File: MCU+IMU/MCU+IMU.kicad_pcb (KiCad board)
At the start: 4 copper layers, 32.8 x 32.8 mm, 21 parts, among them J1 Conn_01x04_Male, SW1 SW_Push, U1 LSM6DSV16XTR, U2 STM32F091RCT6, U3 RN4871, U4 MAX7375AXR405

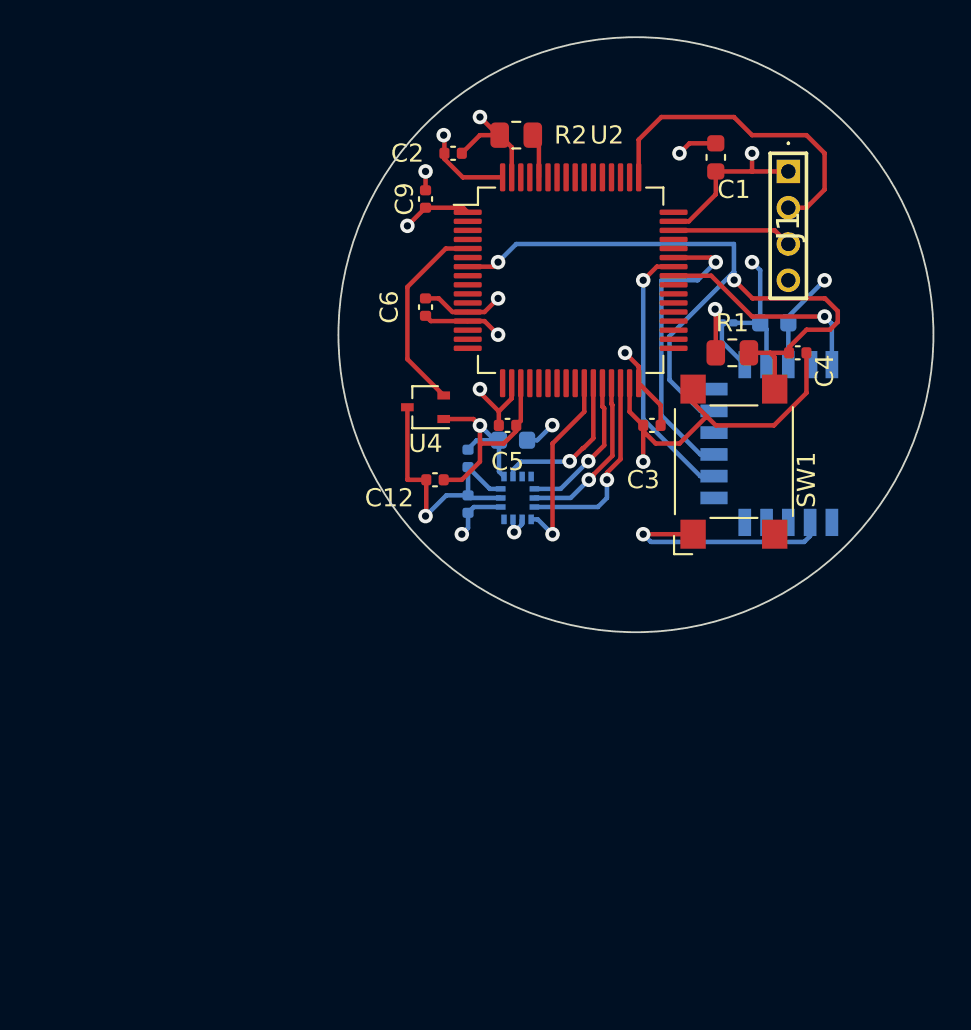
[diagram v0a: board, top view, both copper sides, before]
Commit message: Ordered
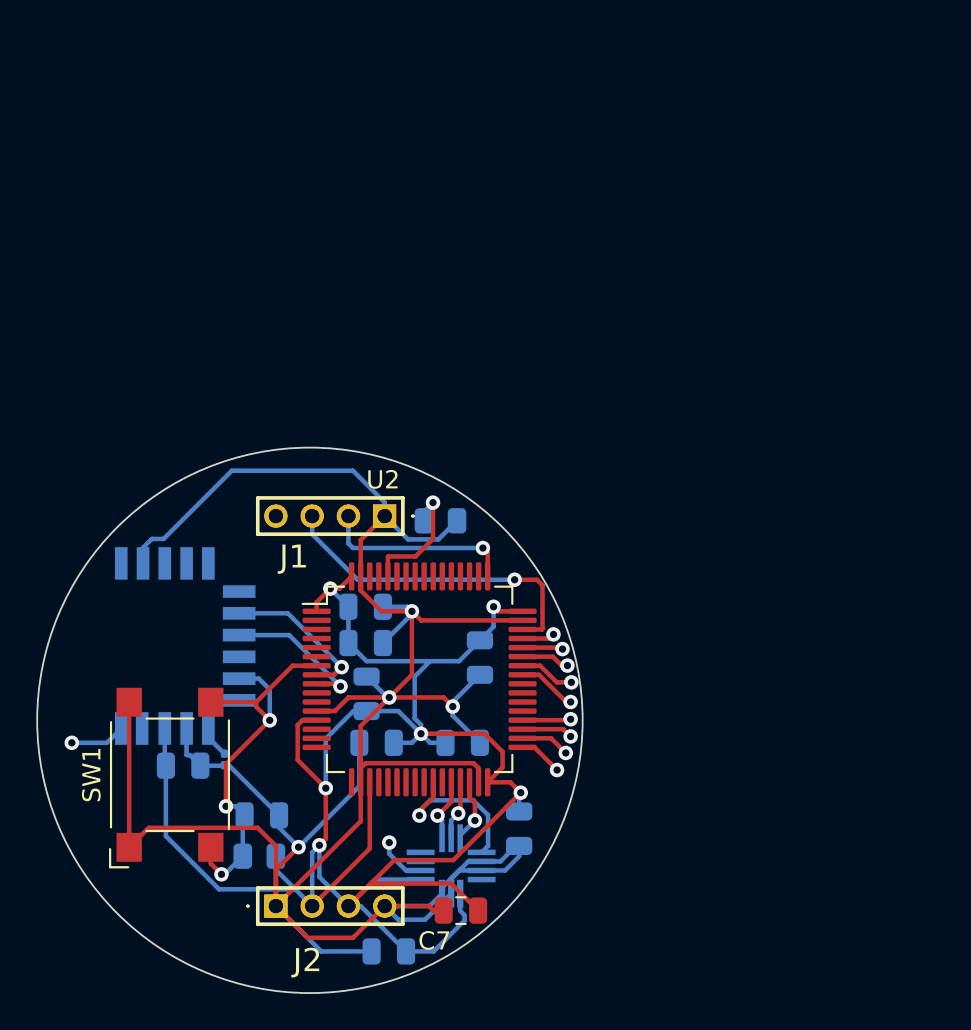
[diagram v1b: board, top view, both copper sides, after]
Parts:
- removed C12: 100n, Capacitor_SMD:C_0402_1005Metric
- removed U4: MAX7375AXR405, Package_TO_SOT_SMD:SOT-323_SC-70
- added J2: Conn_01x04_Male, 4PinConnector:2MMHBS04VT02HTB, F.Cu at (129.8, 113.5)
- C1: footprint Capacitor_SMD:C_0603_1608Metric -> Capacitor_SMD:C_0805_2012Metric; moved to B.Cu
- C10, C11: footprint Capacitor_SMD:C_0603_1608Metric -> Capacitor_SMD:C_0805_2012Metric
- C2, C3, C4, C5, C6, C9: footprint Capacitor_SMD:C_0402_1005Metric -> Capacitor_SMD:C_0805_2012Metric; moved to B.Cu
- C7: footprint Capacitor_SMD:C_0402_1005Metric -> Capacitor_SMD:C_0805_2012Metric; moved to F.Cu
- C8: footprint Capacitor_SMD:C_0402_1005Metric -> Capacitor_SMD:C_0805_2012Metric
- R1, R2: moved to B.Cu
- moved C11 40.7 mm to (124.6, 105.8), turned to 0 degrees
- moved C4 39.0 mm to (129.0, 108.5)
- moved R1 38.1 mm to (128.8, 110.8), turned to 180 degrees
- moved D1 36.7 mm to (126.9, 105.4), turned to 90 degrees
- moved SW1 35.6 mm to (123.9, 106.3)
- moved C1 35.3 mm to (134.8, 101.8), turned to 90 degrees
- moved U3 34.1 mm to (124.7, 99.2), turned to -90 degrees
- moved C9 30.1 mm to (140.1, 104.5), turned to 0 degrees
- moved J1 29.3 mm to (135.8, 92.0), turned to 0 degrees
- moved C10 29.0 mm to (136.0, 116.0), turned to 180 degrees
- moved C2 27.4 mm to (134.7, 99.0)
- moved C7 24.9 mm to (139.9, 113.8), turned to 180 degrees
- moved C6 24.2 mm to (135.3, 104.5), turned to 180 degrees
- moved U2 23.5 mm to (137.7, 101.0)
- moved R2 21.7 mm to (138.8, 92.3), turned to 0 degrees
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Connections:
- U1 pad 9: /IMU_INT -> unconnected-(U1-INT2-Pad9)
- U2 pad 27: /IMU_INT -> unconnected-(U2-PB1-Pad27)
- U2 pad 33: unconnected-(U2-PB12-Pad33) -> /PB12
- U2 pad 34: unconnected-(U2-PB13-Pad34) -> /PB13
- U2 pad 35: unconnected-(U2-PB14-Pad35) -> /PB14
- U2 pad 36: unconnected-(U2-PB15-Pad36) -> /PB15
- U2 pad 41: /MODE_SEL -> /PA8
- U2 pad 42: /USART1_RX -> /PA9
- U2 pad 43: /USART1_TX -> /PA10
- U2 pad 44: unconnected-(U2-PA11-Pad44) -> /PA11
- U2 pad 45: unconnected-(U2-PA12-Pad45) -> /PA12
- U2 pad 48: unconnected-(U2-VDDIO2-Pad48) -> VDD
- U2 pad 5: /SI_OSC -> unconnected-(U2-PF0-Pad5)
- U2 pad 8: unconnected-(U2-PC0-Pad8) -> /USART1_TX
- U2 pad 9: unconnected-(U2-PC1-Pad9) -> /USART1_RX
- U3 pad 16: /MODE_SEL -> unconnected-(U3-P2_0-Pad16)
- U3 pad 7: /USART1_RX -> /USART1_TX
- U3 pad 8: /USART1_TX -> /USART1_RX
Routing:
- net GND: track 85.0 -> 163.2 mm, vias 11 -> 4
- net VDD: track 48.7 -> 123.6 mm, vias 9 -> 6
- net /NRST: track 42.7 -> 24.6 mm, vias 2 -> 3
- net /MODE_SEL: track 12.1 -> 0.00 mm, vias 1 -> 0
- net /SWCLK: track 6.64 -> 18.4 mm, vias 0 -> 1
- net /SI_OSC: track 11.0 -> 0.00 mm
- net /USART1_TX: track 17.1 -> 8.43 mm
- net /IMU_INT: track 8.61 -> 0.00 mm, vias 1 -> 0
- net /SWDIO: track 18.1 -> 10.7 mm, vias 0 -> 1
- net /I2C2_SDA: track 10.8 -> 3.54 mm
- net /USART1_RX: track 14.8 -> 8.13 mm
- net /I2C2_SCL: track 9.30 -> 3.30 mm
- net /IMU Comm En: track 8.31 -> 3.51 mm
- net /BOOT0: track 2.46 -> 7.18 mm, vias 0 -> 1
- net /PA8: track 0.00 -> 3.27 mm, vias 0 -> 1
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- removed copper zone on In1.Cu, net GND
- removed copper zone on In2.Cu, net VDD
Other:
- board size 32.8 x 32.8 mm -> 30.1 x 30.1 mm
- copper layers 4 -> 2
